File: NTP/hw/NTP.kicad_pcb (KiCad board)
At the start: 2 copper layers, 109.3 x 128.5 mm, 94 parts, among them J1 PJ301M-12, J2 PJ301M-12, J3 PJ301M-12, J4 PJ301M-12, J5 PJ301M-12, J6 PJ301M-12, J7 PJ301M-12, J8 PJ301M-12, J9 PJ301M-12, Q1 2N3904, Q10 2N3904, Q11 2N3904, Q12 2N3904, Q13 2N3904, Q14 2N3904, Q15 2N3904, Q16 2N3904, Q17 2N3904, Q18 2N3904, Q2 2N3904, Q3 2N3904, Q4 2N3904, Q5 2N3904, Q6 2N3904, Q7 2N3904, Q8 2N3904, Q9 2N3904

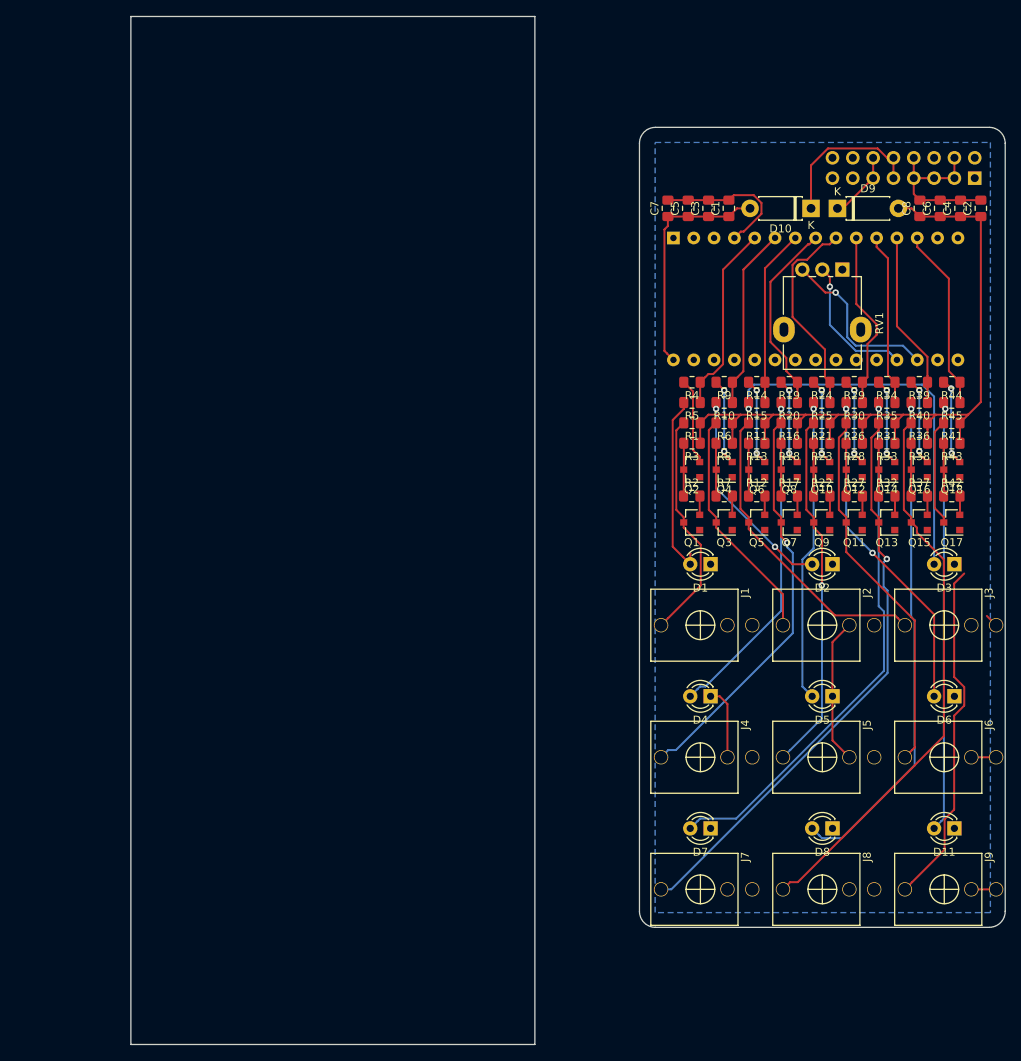
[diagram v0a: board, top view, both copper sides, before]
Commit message: replace and exp adding
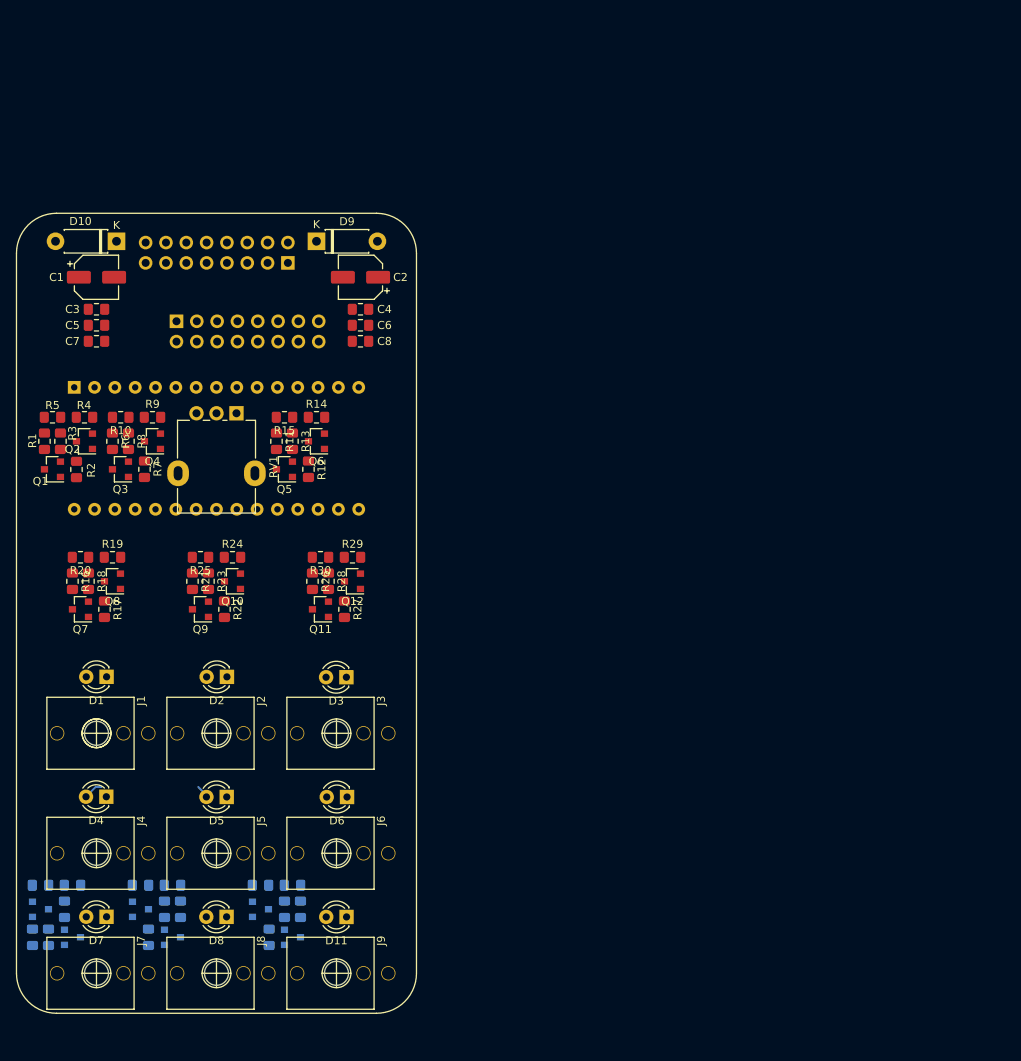
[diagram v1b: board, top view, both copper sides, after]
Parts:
- added EXPANDER: Expander, Connector_PinHeader_2.54mm:PinHeader_2x08_P2.54mm_Vertical, B.Cu at (120.0, 63.5)
- C1, C2: footprint Capacitor_SMD:C_0805_2012Metric_Pad1.15x1.40mm_HandSolder -> Capacitor_SMD:CP_Elec_5x5.3
- C3, C4, C5, C6, C7, C8: value 470n -> 22n
- Q13, Q14, Q15, Q16, Q17, Q18, R31, R32, R33, R34, R35, R36, R37, R38, R39, R40, R41, R42, R43, R44, R45: moved to B.Cu
- ||RED|| --- : renamed from H1
- moved R33 123.4 mm to (102.0, 140.5), turned to 90 degrees
- moved R34 123.1 mm to (103.0, 134.0), turned to 0 degrees
- moved R31 122.9 mm to (104.0, 140.5), turned to 90 degrees
- moved Q14 119.2 mm to (103.0, 137.0), turned to 0 degrees
- moved R35 118.3 mm to (107.0, 134.0), turned to 0 degrees
- moved R39 115.9 mm to (115.5, 134.0)
- moved R32 115.0 mm to (106.0, 137.0), turned to 270 degrees
- moved Q13 114.2 mm to (107.0, 140.5), turned to 0 degrees
- moved Q16 111.8 mm to (115.5, 137.0), turned to 0 degrees
- moved R40 111.2 mm to (119.5, 134.0), turned to 0 degrees
- moved R37 111.0 mm to (116.5, 140.5), turned to 270 degrees
- moved R38 110.9 mm to (118.5, 137.0), turned to 270 degrees
- moved R36 110.6 mm to (120.5, 137.0), turned to 270 degrees
- moved R44 106.9 mm to (130.5, 134.0)
- moved Q15 106.8 mm to (119.5, 140.5), turned to 0 degrees
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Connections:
- A1 pad 23: Net-(A1-Pad23) -> SDA
- A1 pad 24: Net-(A1-Pad24) -> SDC
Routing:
- net 5V: track 104.5 -> 0.00 mm
- net GND: track 74.5 -> 0.00 mm
- net Net-(J7-Pad3): track 72.3 -> 0.00 mm, vias 1 -> 0
- net Net-(J8-Pad3): track 69.7 -> 0.00 mm
- net Net-(D7-Pad2): track 66.2 -> 0.00 mm, vias 1 -> 0
- net Net-(D8-Pad2): track 62.6 -> 0.00 mm, vias 1 -> 0
- net Net-(J9-Pad3): track 57.0 -> 0.00 mm
- net Net-(D11-Pad2): track 53.9 -> 0.00 mm, vias 1 -> 0
- net Net-(J4-Pad3): track 50.5 -> 0.00 mm, vias 1 -> 0
- net Net-(D3-Pad2): track 48.5 -> 0.00 mm, vias 1 -> 0
- net Net-(J6-Pad3): track 46.6 -> 0.00 mm
- net Net-(J5-Pad3): track 45.0 -> 0.00 mm, vias 1 -> 0
- net Net-(D6-Pad2): track 41.3 -> 0.00 mm, vias 2 -> 0
- net Net-(D4-Pad2): track 42.1 -> 2.41 mm, vias 1 -> 0
- net Net-(J3-Pad3): track 38.6 -> 0.00 mm
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- removed copper zone on B.Cu, net GND
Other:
- board size 109.3 x 128.5 mm -> 33 x 33 mm
